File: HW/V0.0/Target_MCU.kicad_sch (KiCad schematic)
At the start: 18 parts, among them SW1 SW-2P, U3 PIC16F877A-I/PT

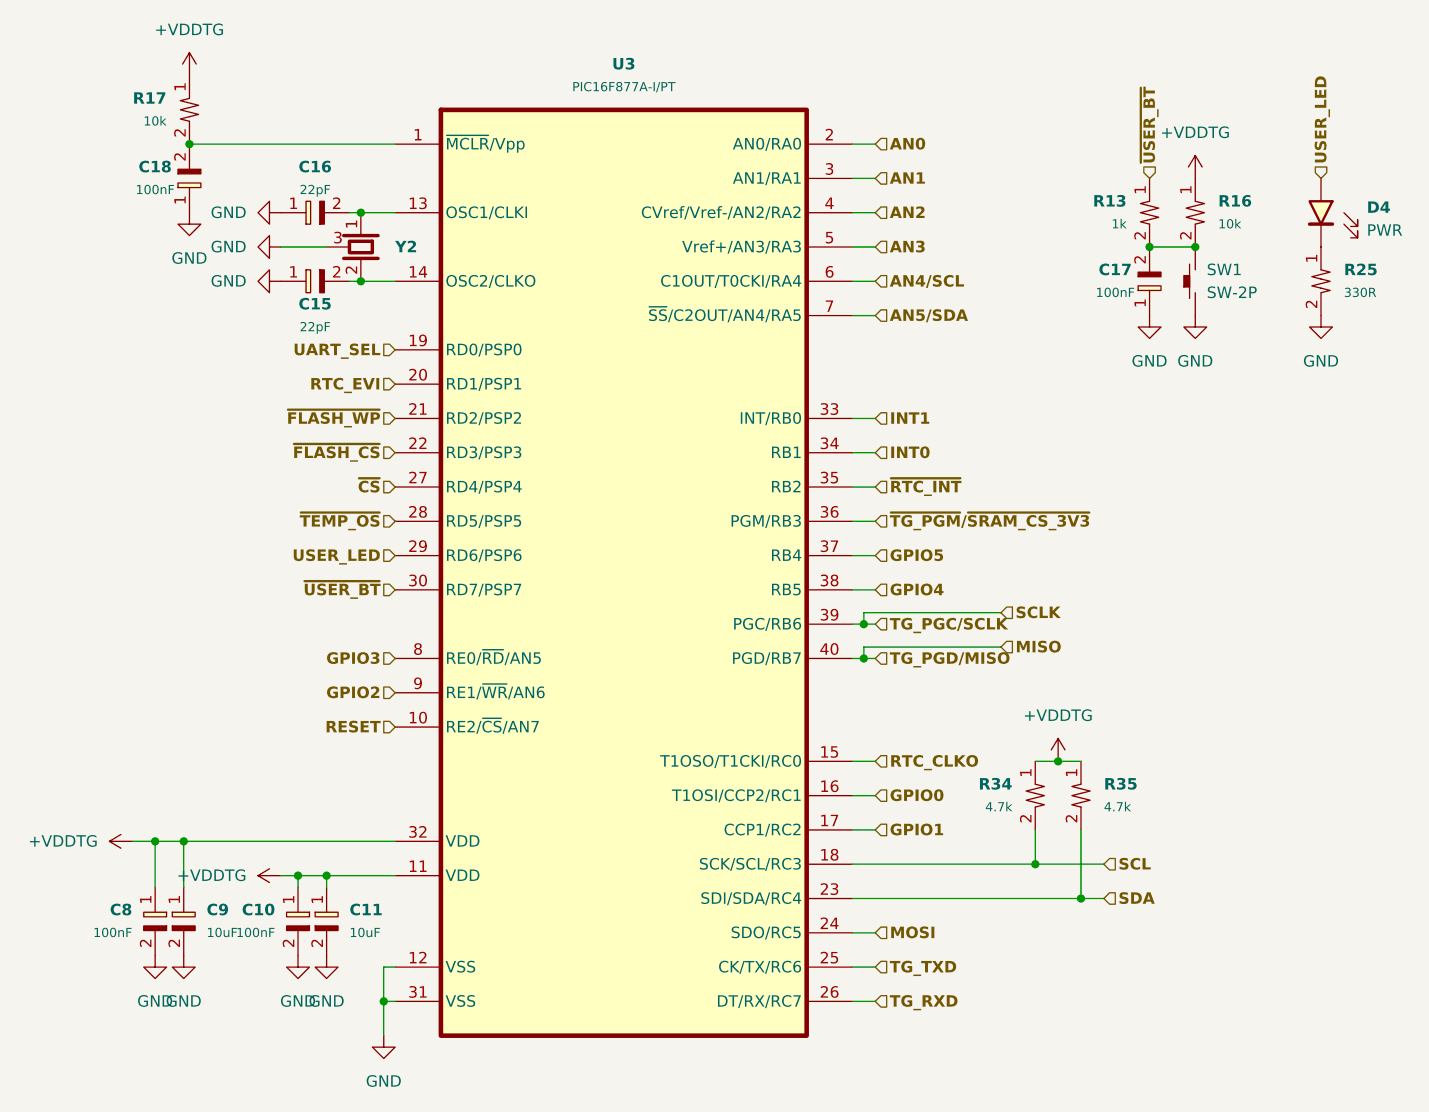
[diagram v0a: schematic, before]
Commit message: PIC16-DevKit-SCH-877 schematic update 1
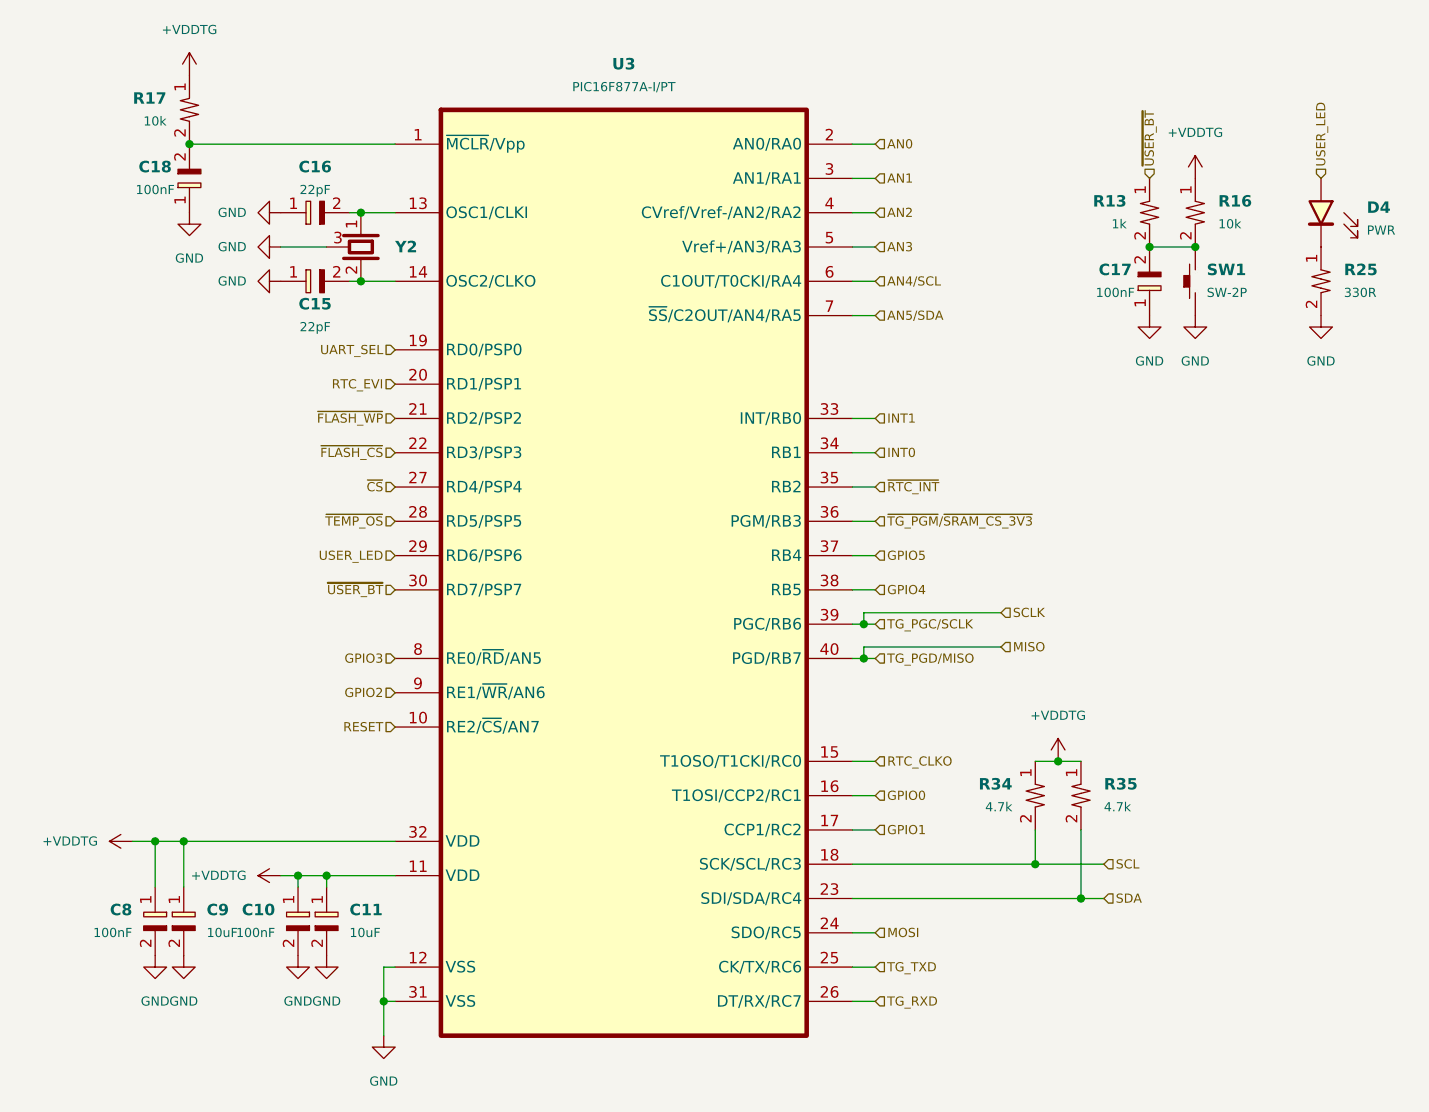
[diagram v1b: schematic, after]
